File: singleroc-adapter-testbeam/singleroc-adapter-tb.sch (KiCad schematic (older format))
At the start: 24 parts, among them J1 CONN_40, J2 CONN-SCSI68, P1 CONN_2

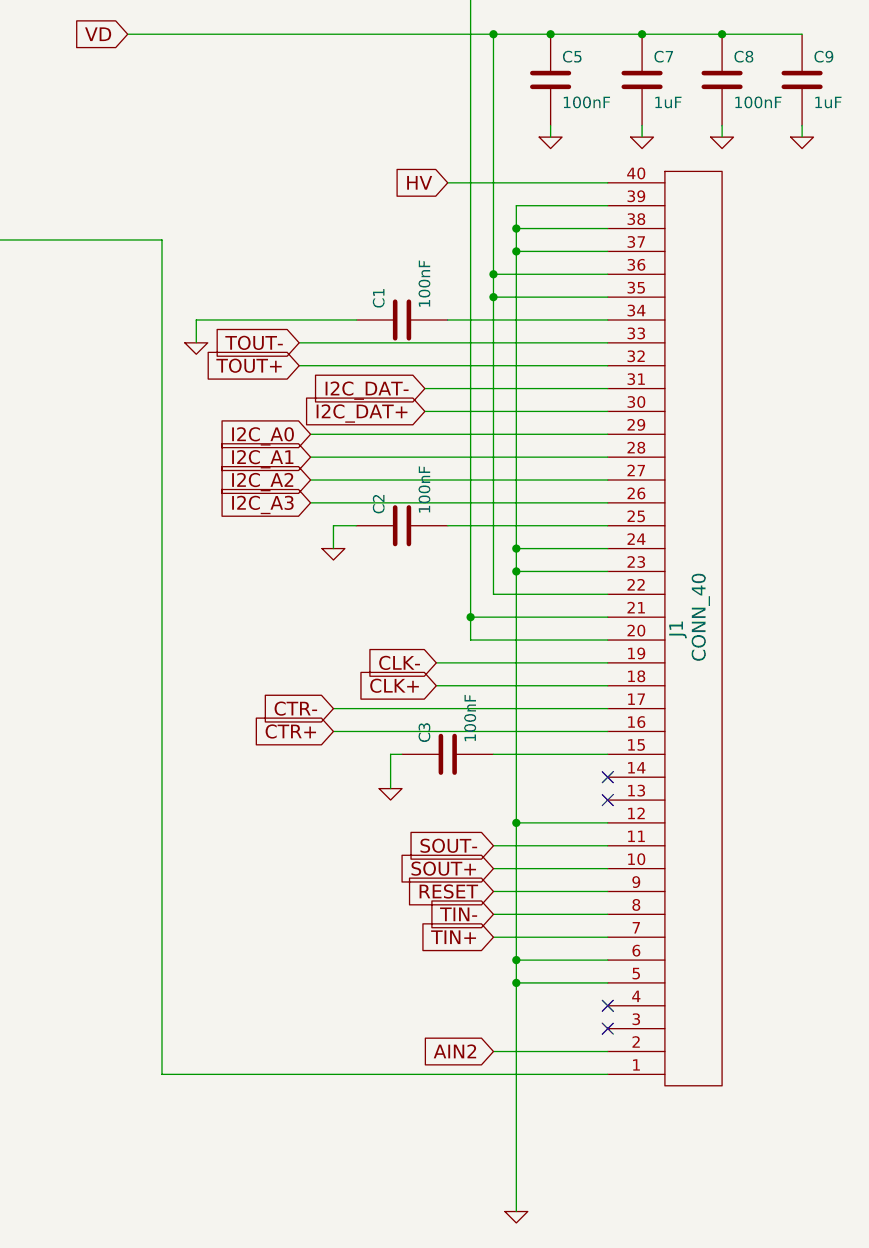
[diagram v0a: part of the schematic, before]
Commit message: updates to the singleroc testbeam adapter
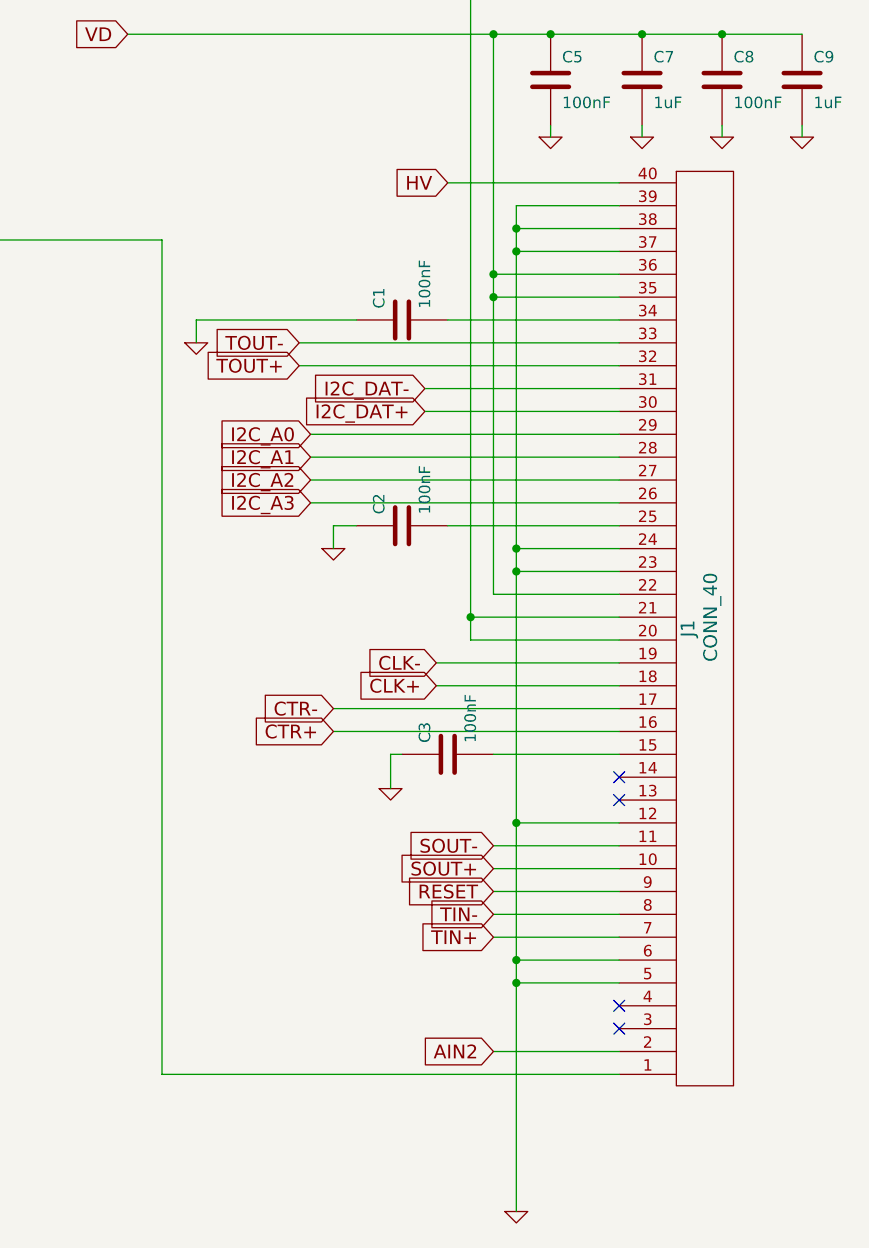
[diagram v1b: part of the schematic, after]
